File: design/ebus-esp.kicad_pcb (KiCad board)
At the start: 2 copper layers, 64.3 x 65.4 mm, 53 parts, among them J1 EBUS, J2 USB_B_Micro, J3 UART, J4 PROG, J5 PINS, J6 PWR, J7 UART, J8 Measurements, Q1 BC817, U1 LM393, U2 LTV-357T, U3 L7805, U4 LTV-357T, U5 AMS1117-3.3, U6 ESP-12F

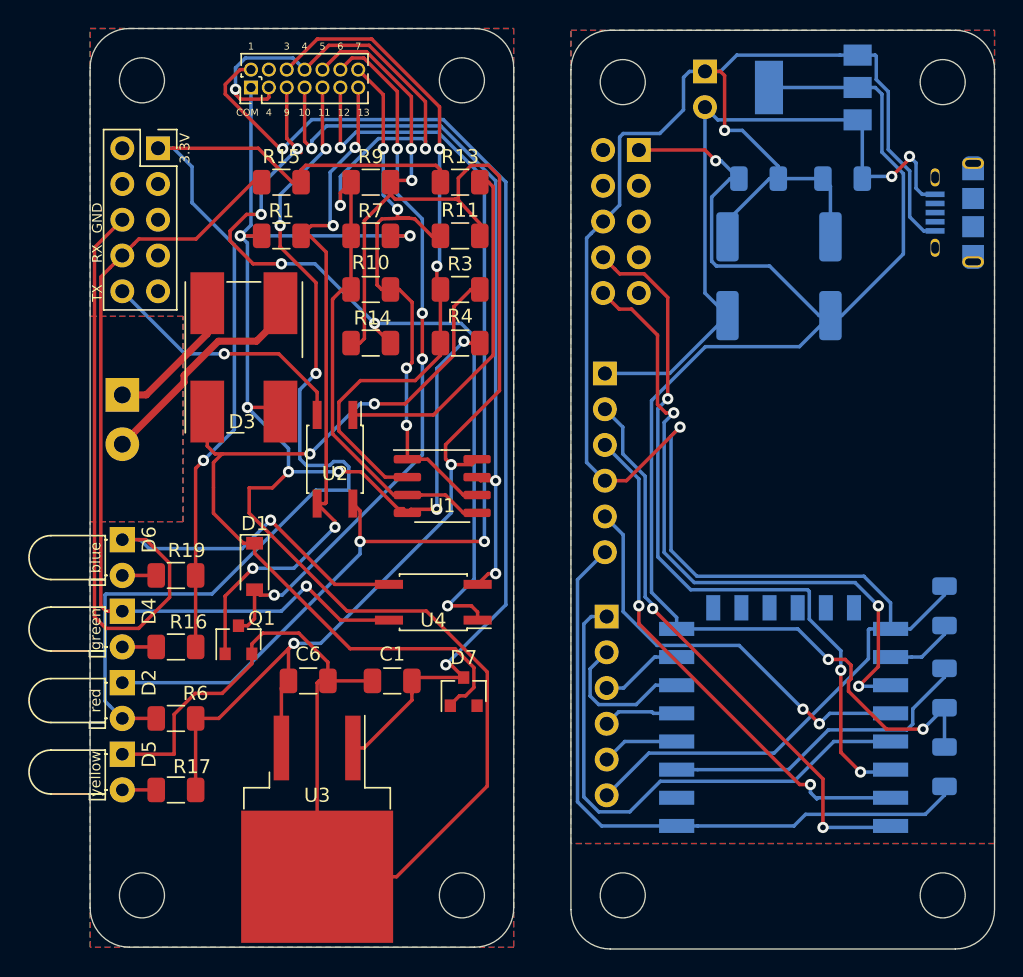
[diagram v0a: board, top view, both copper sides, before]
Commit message: Raspberry board update
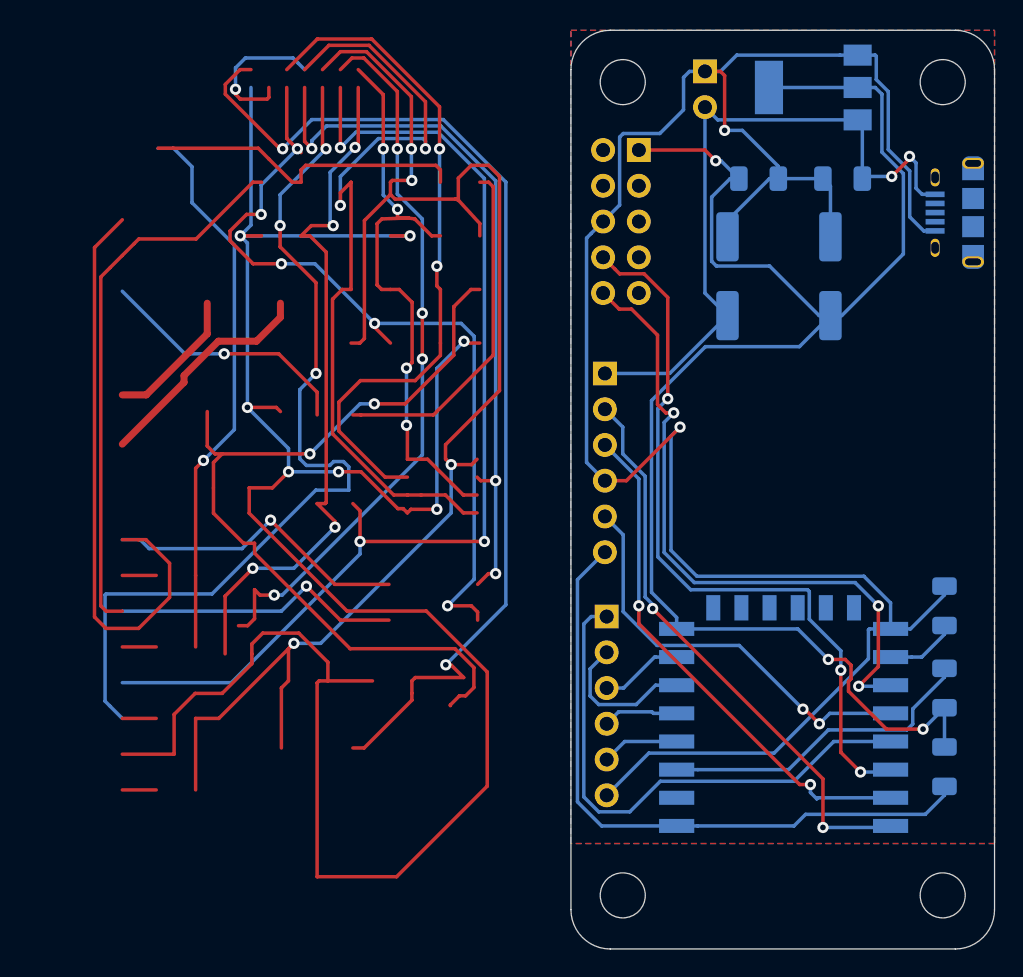
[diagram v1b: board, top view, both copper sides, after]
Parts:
- removed C1: 330nF, Capacitor_SMD:C_1206_3216Metric
- removed C6: 100nF, Capacitor_SMD:C_1206_3216Metric
- removed D1: 1N4737A 7.5V, Diode_SMD:D_SOD-123
- removed D2: TX red, LED_THT:LED_D3.0mm_Horizontal_O1.27mm_Z2.0mm
- removed D3: DF10M, Diode_SMD:Diode_Bridge_Bourns_CD-DF4xxS
- removed D4: RX green, LED_THT:LED_D3.0mm_Horizontal_O1.27mm_Z2.0mm
- removed D5: EBUS yellow, LED_THT:LED_D3.0mm_Horizontal_O1.27mm_Z2.0mm
- removed D6: ESP blue, LED_THT:LED_D3.0mm_Horizontal_O1.27mm_Z2.0mm
- removed D7: 1N914, Package_TO_SOT_SMD:SOT-23
- removed H1, H2, H3, H4: MountingHole, MountingHole:MountingHole_3.2mm_M3
- removed J1: EBUS, TerminalBlock_4Ucon:TerminalBlock_4Ucon_1x02_P3.50mm_Horizontal
- removed J3: UART, Connector_PinSocket_2.54mm:PinSocket_2x05_P2.54mm_Vertical
- removed J8: Measurements, Connector_PinHeader_1.27mm:PinHeader_2x07_P1.27mm_Vertical
- removed Q1: BC817, Package_TO_SOT_SMD:SOT-23
- removed R1, R16: 220, Resistor_SMD:R_1206_3216Metric
- removed R10: 220k, Resistor_SMD:R_1206_3216Metric
- removed R11, R17, R19: 10k, Resistor_SMD:R_1206_3216Metric
- removed R13, R6: 470, Resistor_SMD:R_1206_3216Metric
- removed R14: 390, Resistor_SMD:R_1206_3216Metric
- removed R15: 820, Resistor_SMD:R_1206_3216Metric
- removed R3: 100k, Resistor_SMD:R_1206_3216Metric
- removed R4: 22k, Resistor_SMD:R_1206_3216Metric
- removed R7: 15k, Resistor_SMD:R_1206_3216Metric
- removed R9: 18k, Resistor_SMD:R_1206_3216Metric
- removed U1: LM393, Package_SO:SOIC-8_3.9x4.9mm_P1.27mm
- removed U2, U4: LTV-357T, Package_SO:SO-4_4.4x3.6mm_P2.54mm
- removed U3: L7805, Package_TO_SOT_SMD:TO-263-2
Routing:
- removed copper zone on B.Cu, net (none)
- removed copper zone on F.Cu, net GNDD
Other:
- board size 64.3 x 65.4 mm -> 30.1 x 65.3 mm
- board text removed: "1"
- board text removed: "10"
- board text removed: "11"
- board text removed: "12"
- board text removed: "13"
- board text removed: "3"
- board text removed: "4"
- board text removed: "5"
- board text removed: "6"
- board text removed: "7"
- board text removed: "9"
- board text removed: "COM"
- board text removed: "EBUS"
- board text removed: "blue"
- board text removed: "green"
- board text removed: "red"
- board text removed: "smart home"
- board text removed: "yellow"
